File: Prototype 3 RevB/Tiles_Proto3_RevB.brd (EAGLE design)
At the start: 46 x 46 mm, 63 parts, among them Q1 DMG3415U-7, T2 MF-DSC-SOT233-MMBT3904, U1 MDBT42Q, U2 AP2112, U3 ADXL345, U4 CAP1188, U5 DRV2605L, X1 32.768

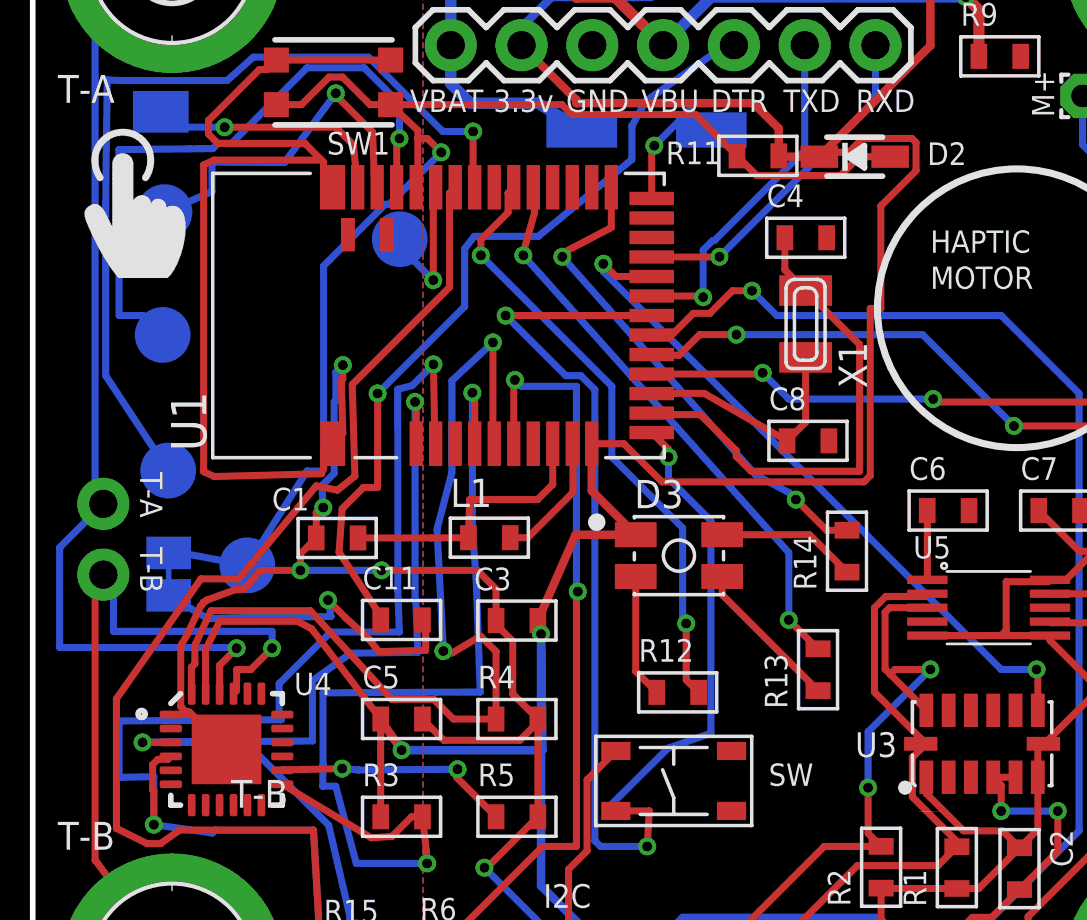
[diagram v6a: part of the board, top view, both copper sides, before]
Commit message: ready for ready for prod
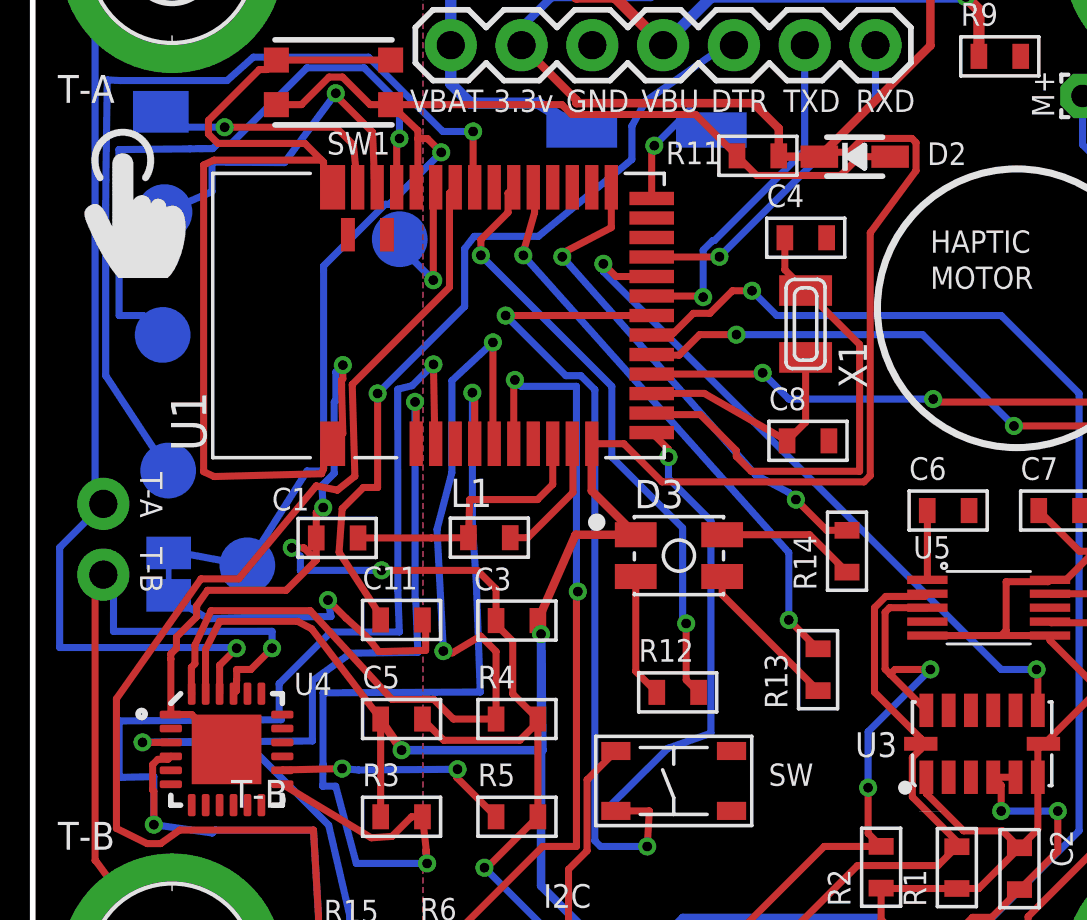
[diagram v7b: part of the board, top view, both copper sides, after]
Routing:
- net GND: track 145.2 -> 145.8 mm
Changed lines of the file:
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@@
 <wire x1="15.954053125" y1="-26.844053125" x2="12.5181" y2="-26.844053125" width="0.254" layer="1"/>
 <via x="12.5181" y="-26.844053125" extent="1-16" drill="0.35"/>
-<wire x1="12.5181" y1="-26.844053125" x2="9.604053125" y2="-26.844053125" width="0.254" layer="16"/>
+<wire x1="9.604053125" y1="-26.844053125" x2="12.5181" y2="-26.844053125" width="0.254" layer="16"/>
 <wire x1="9.604053125" y1="-26.844053125" x2="9.604" y2="-26.844" width="0.254" layer="16"/>
-<via x="9.604" y="-26.844" extent="1-16" drill="0.35"/>
-<wire x1="9.604" y1="-26.844" x2="9.604" y2="-26.2505" width="0.254" layer="1"/>
-<wire x1="9.604" y1="-26.2505" x2="10.173" y2="-25.6815" width="0.254" layer="1"/>
 <wire x1="16.6249" y1="-27.5149" x2="15.954053125" y2="-26.844053125" width="0.254" layer="1"/>
-<wire x1="5.3114" y1="-29.5872" x2="5.3368" y2="-29.511" width="0.254" layer="1"/>
-<wire x1="6.9556" y1="-33.2678" x2="5.6096" y2="-31.9218" width="0.254" layer="1"/>
-<wire x1="5.6096" y1="-31.9218" x2="5.50139375" y2="-31.9218" width="0.254" layer="1"/>
-<wire x1="5.50139375" y1="-31.9218" x2="5.3114" y2="-31.73180625" width="0.254" layer="1"/>
-<wire x1="5.3114" y1="-31.73180625" x2="5.3114" y2="-29.5872" width="0.254" layer="1"/>
-<wire x1="6.01718125" y1="-28.13398125" x2="6.081359375" y2="-28.069803125" width="0.254" layer="1"/>
-<wire x1="6.081359375" y1="-28.069803125" x2="6.119765625" y2="-27.987575" width="0.254" layer="1"/>
-<wire x1="6.119765625" y1="-27.987575" x2="6.1885875" y2="-27.962575" width="0.254" layer="1"/>
-<wire x1="6.1885875" y1="-27.962575" x2="6.2403625" y2="-27.9108" width="0.254" layer="1"/>
-<wire x1="7.55123125" y1="-27.5298" x2="7.56196875" y2="-27.5190625" width="0.254" layer="1"/>
-<wire x1="7.56196875" y1="-27.5190625" x2="7.5771125" y2="-27.518015625" width="0.254" layer="1"/>
-<wire x1="7.5771125" y1="-27.518015625" x2="7.672078125" y2="-27.408953125" width="0.254" layer="1"/>
-<wire x1="7.672078125" y1="-27.408953125" x2="7.7744125" y2="-27.30661875" width="0.254" layer="1"/>
-<wire x1="5.3368" y1="-29.511" x2="5.54020625" y2="-29.15519375" width="0.254" layer="1"/>
-<wire x1="5.54020625" y1="-29.15519375" x2="6.01718125" y2="-28.13398125" width="0.254" layer="1"/>
-<wire x1="7.7744125" y1="-27.30661875" x2="8.1772375" y2="-26.844" width="0.254" layer="1"/>
-<wire x1="8.1772375" y1="-26.844" x2="9.604" y2="-26.844" width="0.254" layer="1"/>
-<wire x1="7.406909375" y1="-27.539771875" x2="7.55123125" y2="-27.5298" width="0.254" layer="1"/>
-<wire x1="6.2403625" y1="-27.9108" x2="7.261746875" y2="-27.539771875" width="0.254" layer="1"/>
-<wire x1="7.261746875" y1="-27.539771875" x2="7.406909375" y2="-27.539771875" width="0.254" layer="1"/>
 <wire x1="18.1249" y1="-32.2931" x2="18.1249" y2="-35.6858" width="0.254" layer="1"/>
 <wire x1="20.925" y1="-33.325" x2="19.891" y2="-34.359" width="0.254" layer="1"/>
@@
 <wire x1="15" y1="-45" x2="14.75" y2="-44.75" width="0.254" layer="1"/>
 <wire x1="14.75" y1="-44.75" x2="14.75" y2="-43.8" width="0.254" layer="1"/>
+<wire x1="4.9556" y1="-32.0178" x2="4.9556" y2="-30.0254" width="0.254" layer="1"/>
+<wire x1="4.9556" y1="-30.0254" x2="4.953" y2="-30.0228" width="0.254" layer="1"/>
+<wire x1="4.953" y1="-30.0228" x2="4.953" y2="-29.845" width="0.254" layer="1"/>
+<wire x1="4.953" y1="-29.845" x2="5.1562" y2="-29.6418" width="0.254" layer="1"/>
+<wire x1="5.1562" y1="-29.6418" x2="5.1562" y2="-29.2354" width="0.254" layer="1"/>
+<wire x1="5.1562" y1="-29.2354" x2="5.8706375" y2="-28.5209625" width="0.254" layer="1"/>
+<wire x1="5.8706375" y1="-28.5209625" x2="5.883103125" y2="-28.49426875" width="0.254" layer="1"/>
+<wire x1="5.883103125" y1="-28.49426875" x2="5.883103125" y2="-28.113215625" width="0.254" layer="1"/>
+<wire x1="5.883103125" y1="-28.113215625" x2="6.2738" y2="-27.559" width="0.254" layer="1"/>
+<wire x1="6.2738" y1="-27.559" x2="9.0932" y2="-27.559" width="0.254" layer="1"/>
+<wire x1="10.173" y1="-25.6815" x2="10.173" y2="-26.4792" width="0.254" layer="1"/>
+<wire x1="9.0932" y1="-27.559" x2="10.173" y2="-26.4792" width="0.254" layer="1"/>
+<wire x1="10.173" y1="-26.4792" x2="9.7288" y2="-26.035" width="0.254" layer="1"/>
+<wire x1="9.7288" y1="-26.035" x2="9.2964" y2="-26.035" width="0.254" layer="1"/>
+<via x="9.2964" y="-26.035" extent="1-16" drill="0.35"/>
+<wire x1="9.2964" y1="-26.035" x2="9.604053125" y2="-26.342653125" width="0.254" layer="16"/>
+<wire x1="9.604053125" y1="-26.342653125" x2="9.604053125" y2="-26.844053125" width="0.254" layer="16"/>
 </signal>
 <signal name="RESET">
@@
 <wire x1="21.2107875" y1="-22.3" x2="22.5797875" y2="-23.669" width="0.254" layer="1"/>
 <wire x1="22.5797875" y1="-23.669" x2="29.82781875" y2="-23.669" width="0.254" layer="1"/>
-<wire x1="30.051" y1="-23.44581875" x2="30.051" y2="-17.446" width="0.254" layer="1"/>
-<wire x1="30.051" y1="-17.446" x2="30.432" y2="-17.446" width="0.254" layer="1"/>
+<wire x1="30.051" y1="-23.44581875" x2="30.051" y2="-18.4112" width="0.254" layer="1"/>
 <wire x1="31.694" y1="-12.5052125" x2="31.694" y2="-11.4947875" width="0.254" layer="1"/>
 <wire x1="31.694" y1="-11.4947875" x2="31.5452125" y2="-11.346" width="0.254" layer="1"/>
@@
 <wire x1="31.5452125" y1="-11.346" x2="29.77439375" y2="-11.346" width="0.254" layer="1"/>
 <wire x1="29.77439375" y1="-11.346" x2="29.27889375" y2="-11.8415" width="0.254" layer="1"/>
-<wire x1="30.432" y1="-17.446" x2="30.432" y2="-13.7672125" width="0.254" layer="1"/>
-<wire x1="30.432" y1="-13.7672125" x2="31.694" y2="-12.5052125" width="0.254" layer="1"/>
+<wire x1="30.051" y1="-18.4112" x2="30.051" y2="-14.7324125" width="0.254" layer="1"/>
+<wire x1="30.051" y1="-14.7324125" x2="31.694" y2="-12.5052125" width="0.254" layer="1"/>
 </signal>
 <signal name="N$11">

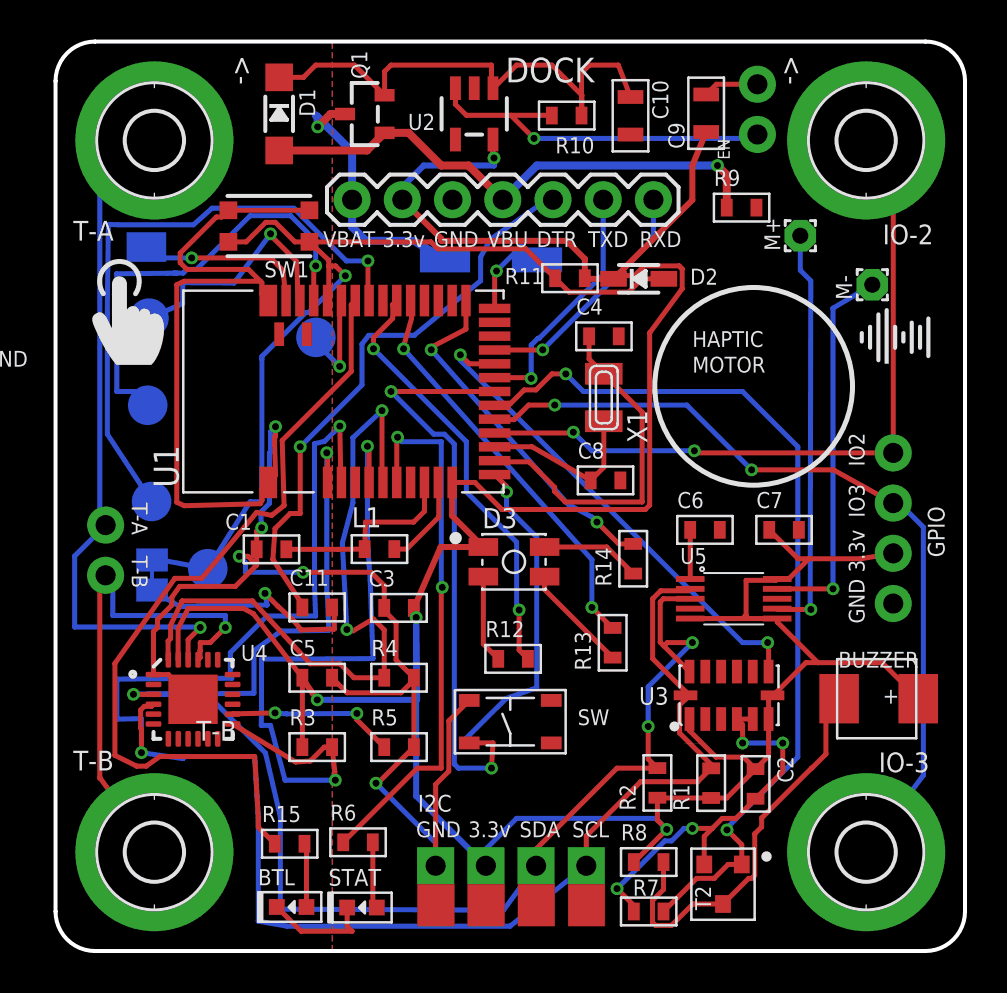
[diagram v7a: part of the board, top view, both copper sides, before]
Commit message: ready for prod
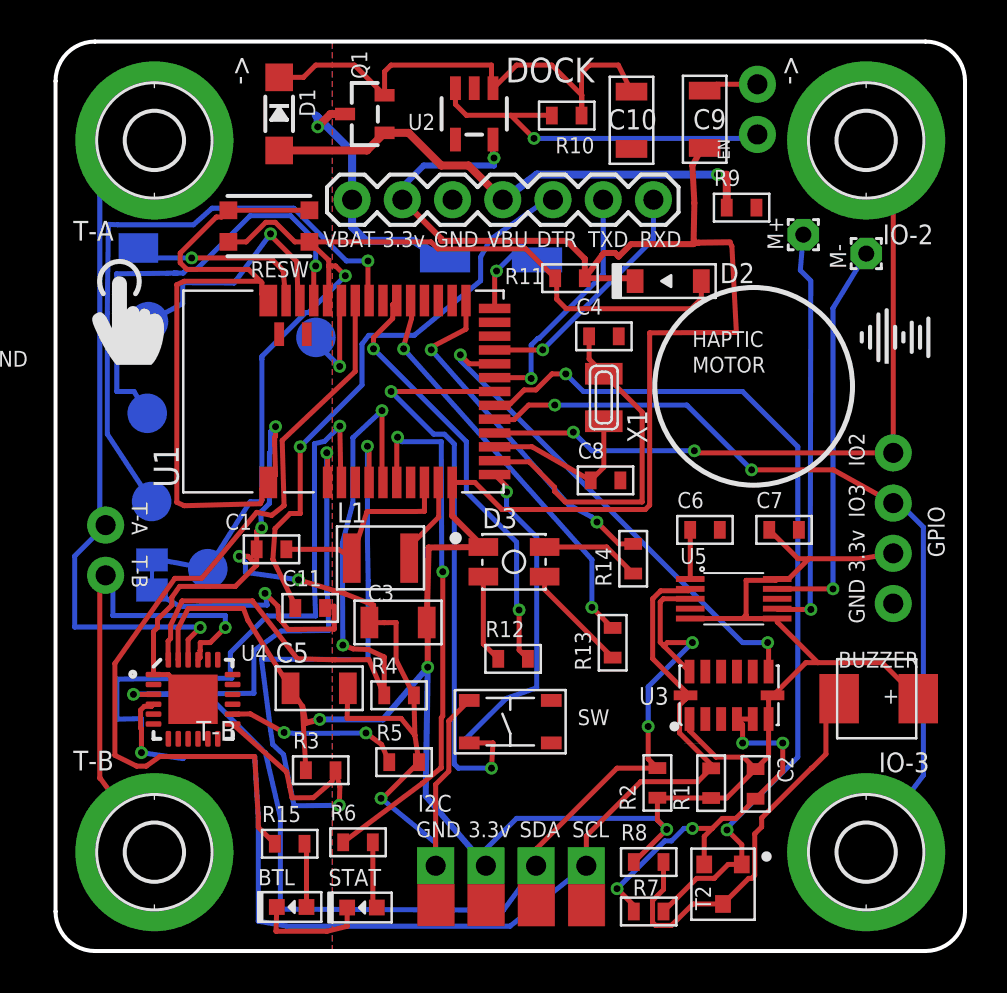
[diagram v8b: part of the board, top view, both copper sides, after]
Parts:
- BTL: value MF-LED-0603-RED -> RED
- C10, C9: device MF_Passives:C0805 -> MF_Passives:C1206
- C2: value 100nF -> 0.1uF
- C3, C5: device MF_Passives:C0603 -> MF_Passives:C1206
- D2: device microbuilder2:SOD-323 -> MF_Discrete_Semiconductor:SOD-123
- D3: value MF-LED-3228-RGB -> RGBLED
- L1: device MF_Passives:L0603 -> MF_Passives:L1210
- STAT: value MF-LED-0603-RED -> WHITE
- SW: value MF-SW-TACT-4.2MM -> SW
- T2: value MF-DSC-SOT233-MMBT3904 -> MMBT3904
- moved M- 1.60 mm to (41.0, -10.7)
- moved D2 1.50 mm to (31.0, -12.1)
- moved R3 1.18 mm to (13.4, -36.9)
- moved R4 0.89 mm to (17.4, -33.1)
- moved R5 0.80 mm to (17.6, -36.4)
- moved C3 0.74 mm to (17.3, -29.4)
- moved C5 0.54 mm to (13.3, -32.7)
- moved L1 0.46 mm to (16.4, -26.1)
- moved FRST 0.41 mm to (4.19, -10.4)
- moved SWCLK 0.41 mm to (4.64, -18.8)
- moved C11 0.36 mm to (12.9, -28.6)
- moved C9 0.31 mm to (32.8, -3.93)
- moved C10 0.23 mm to (29.1, -3.98)
- moved SWDIO 0.18 mm to (4.70, -14.2)
- moved M+ 0.16 mm to (37.8, -9.77)
- renumbered SW1 to RESW
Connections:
- net 3.3V: now also D2.CATHODE; no longer D2.C
- net RESET: now also D2.ANODE; no longer D2.A
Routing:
- net 3.3V: track 162.6 -> 169.1 mm
- net RESET: track 49.5 -> 53.1 mm
- net CAP-INT: track 35.0 -> 37.8 mm
- net CAP-RES: track 35.2 -> 36.4 mm
- net N$7: track 19.3 -> 20.2 mm
- net N$20: track 12.2 -> 12.9 mm
